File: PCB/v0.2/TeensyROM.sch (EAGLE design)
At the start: 23 parts, among them J1 C64-EXPANSION-PORT, J2 3 pin Header, U1 TEENSY41, U2 74LCV245, U3 74LCV245, U4 74LCV245, U5 74LCV245, U6 74LVC07, X2 SI-50170

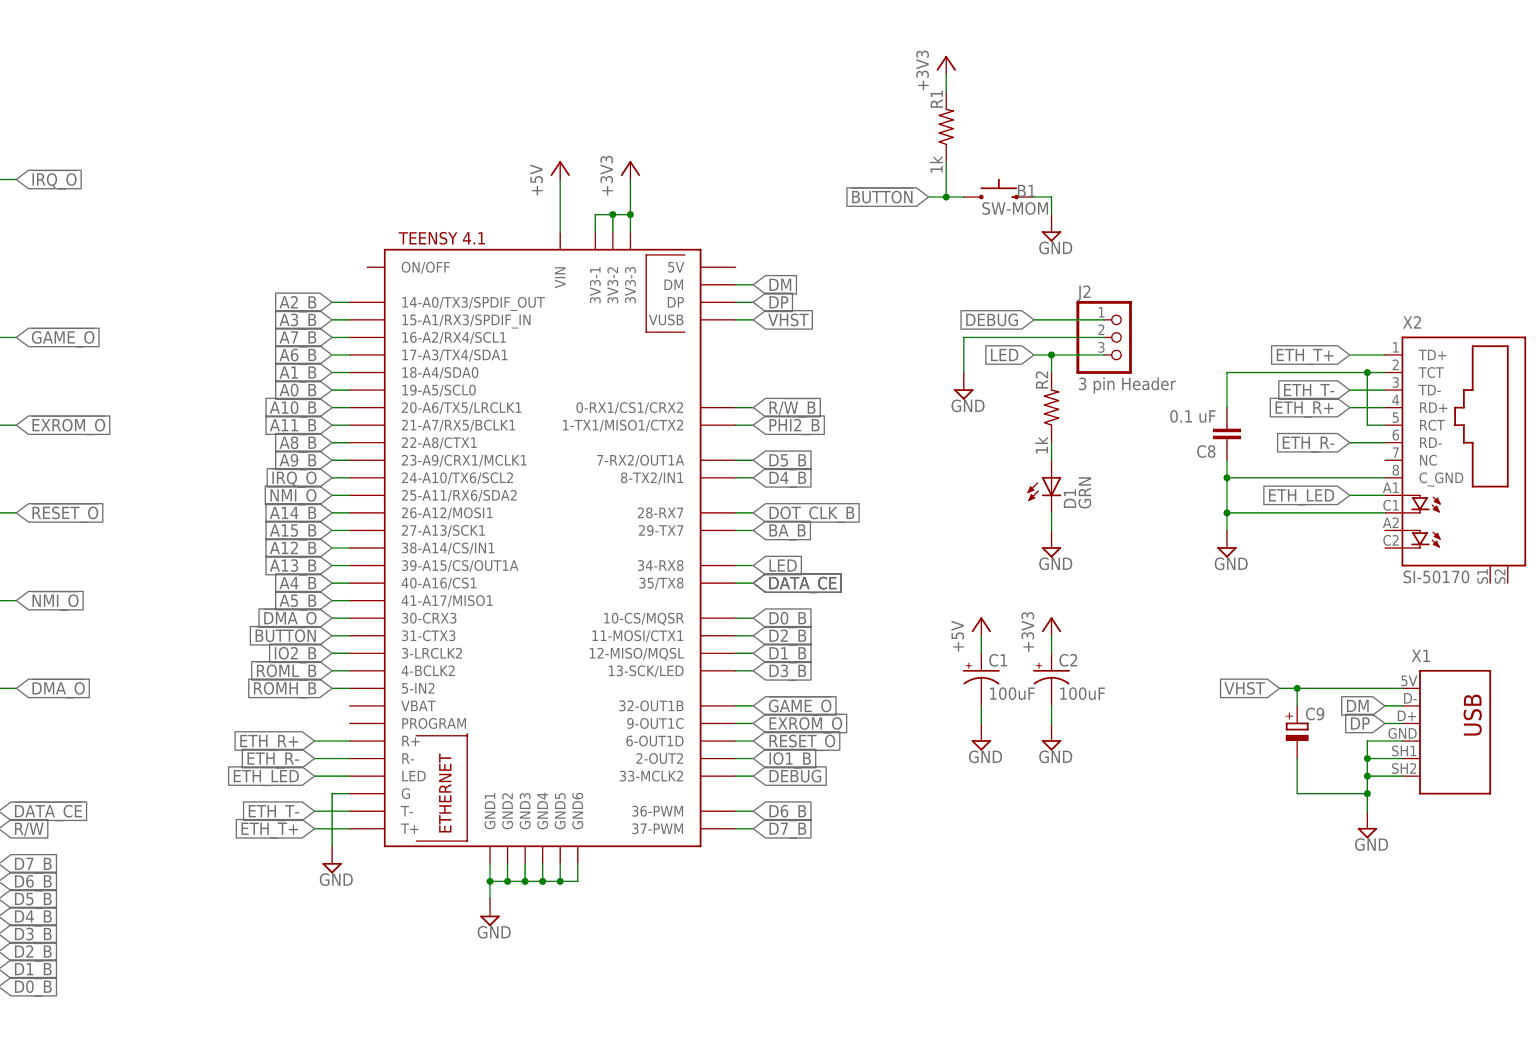
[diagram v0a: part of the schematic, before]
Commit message: PCB 0.2 progress (not yet complete)
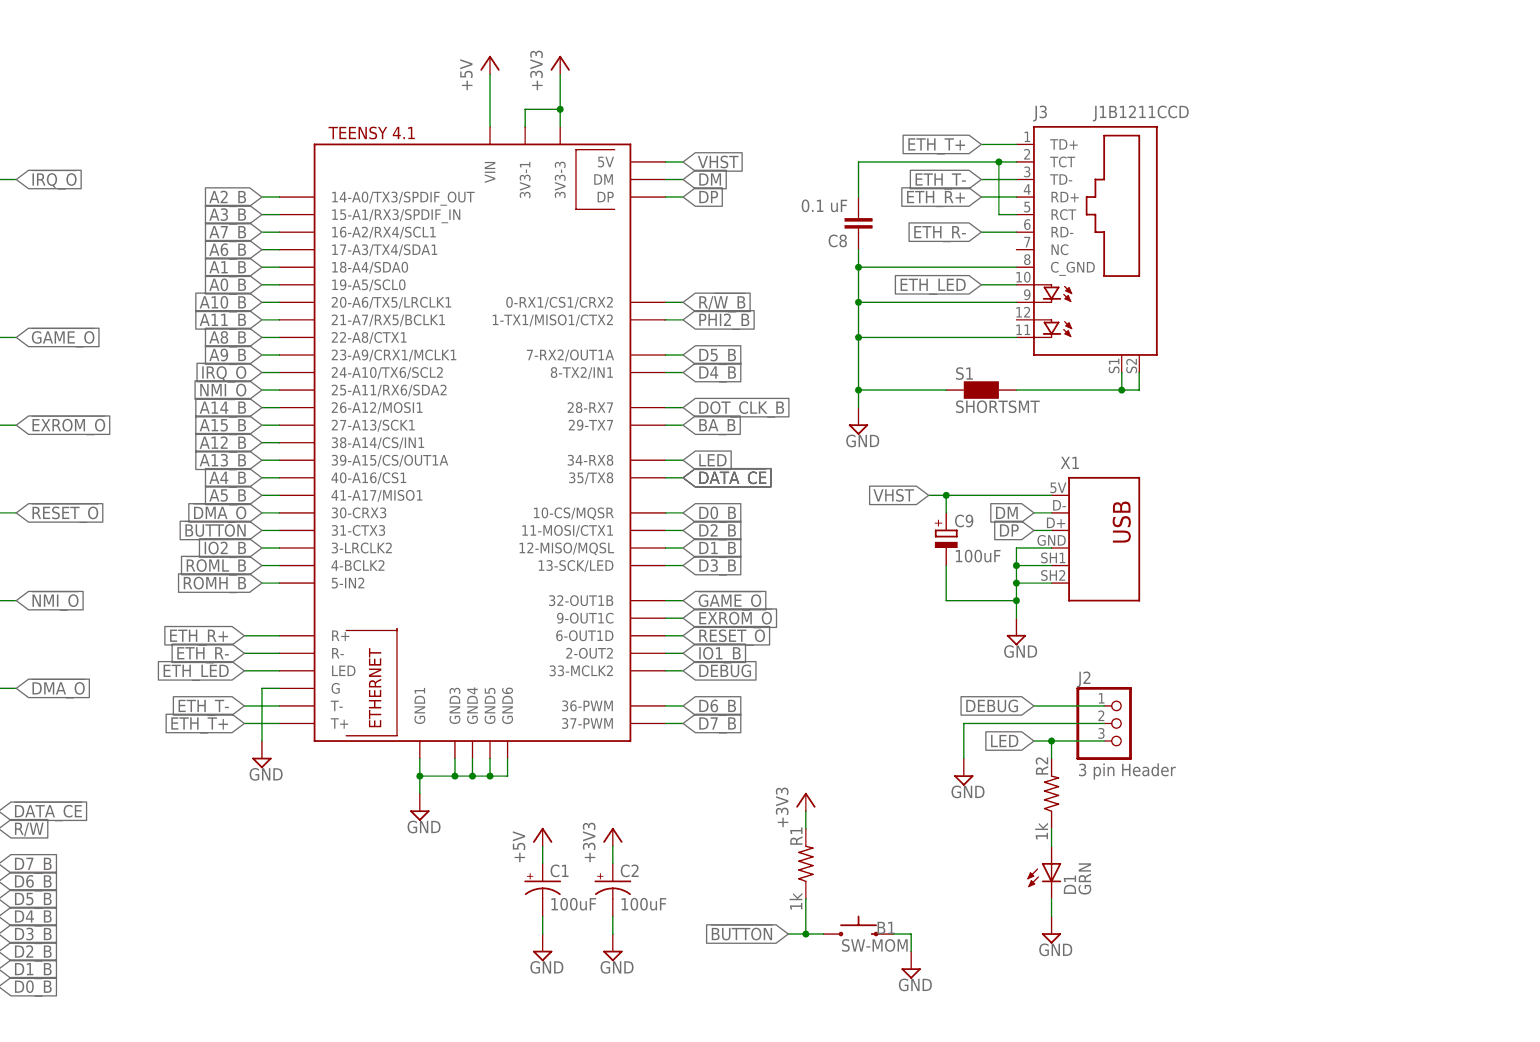
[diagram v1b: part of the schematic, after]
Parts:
- removed X2: SI-50170, TeensyROM:SI-50170
- added J3: J1B1211CCD, TeensyROM:J1B1211CCD
- added S1: SHORTSMT, AudioLooper:SHORTSMT
- C9: value (none) -> 100uF
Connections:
- net N$1 renamed LED_R
- removed net N$2: C8.2, X2.RCT, X2.TCT
- new net ETH_CT: C8.2, J3.RCT, J3.TCT
- new net ETH_SH: J3.S1, J3.S2, S1.2
- net +3V3: no longer U1.3V3-2
- net DM: now also X1.2
- net DP: now also X1.3
- net ETH_LED: now also J3.A; no longer X2.A
- net ETH_R+: now also J3.RD+; no longer X2.RD+
- net ETH_R-: now also J3.RD-; no longer X2.RD-
- net ETH_T+: now also J3.TD+; no longer X2.TD+
- net ETH_T-: now also J3.TD-; no longer X2.TD-
- net GND: now also J3.C, J3.C1, J3.C_GND, S1.1, X1.6; no longer U1.GND2, X2.C, X2.C_GND
- net VHST: now also U1.5V, X1.1; no longer U1.VUSB
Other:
- moved on the sheet: B1, C1, C2, C8, C9, D1, J2, R1, R2, X1
